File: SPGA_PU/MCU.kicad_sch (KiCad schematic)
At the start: 5 parts, among them U19 ESP32-S3-WROOM-1

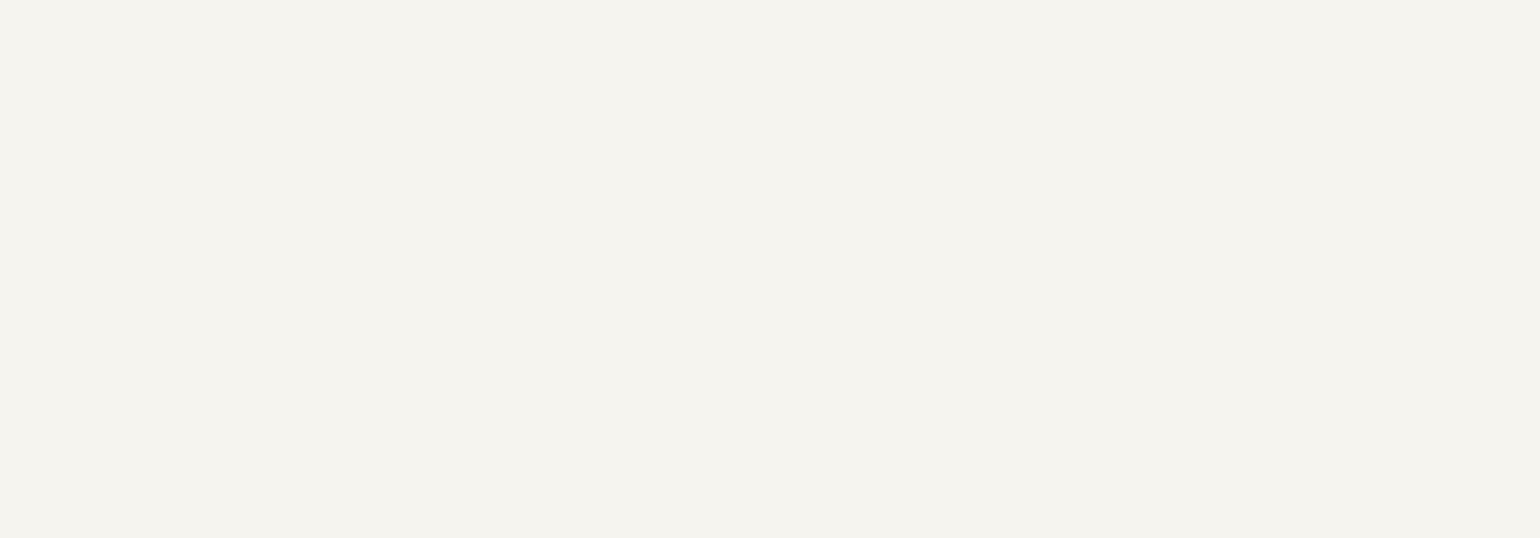
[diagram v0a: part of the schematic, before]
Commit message: thibgs
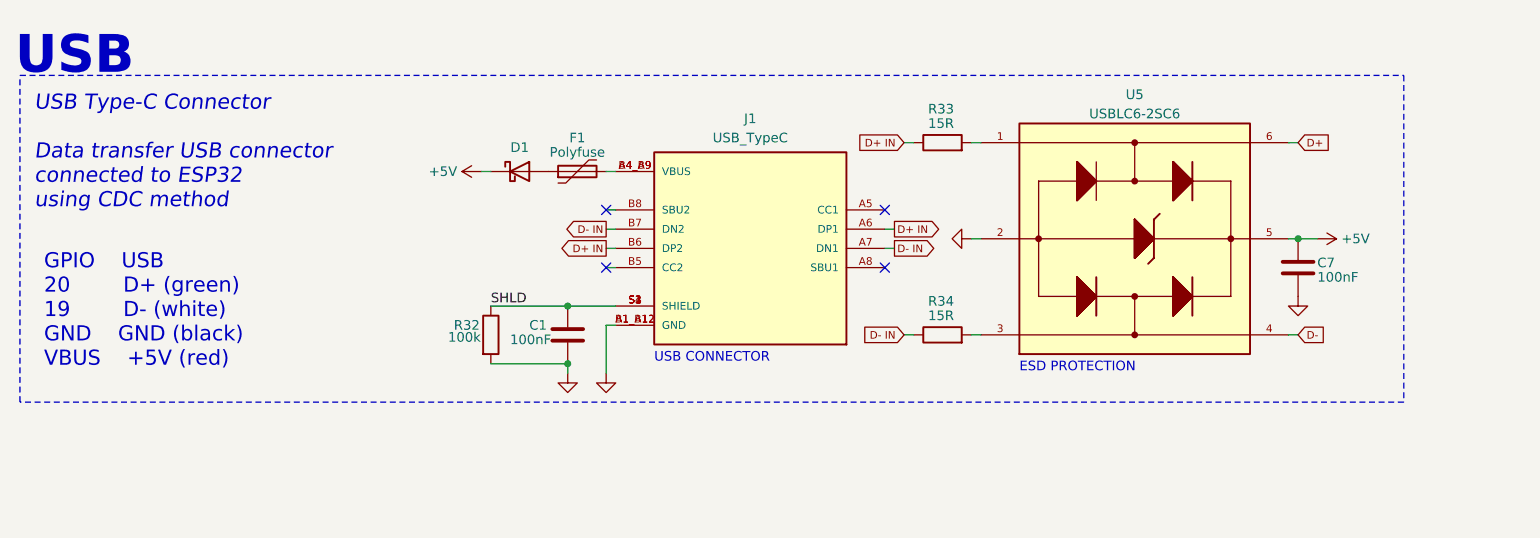
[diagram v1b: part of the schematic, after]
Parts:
- added C1, C7: 100nF, Capacitor_SMD:C_0805_2012Metric_Pad1.18x1.45mm_HandSolder, symbol Device:C
- added D1: D_Schottky, Diode_SMD:D_1206_3216Metric_Pad1.42x1.75mm_HandSolder, symbol Device:D_Schottky
- added F1: Polyfuse, Fuse:Fuse_0805_2012Metric, symbol Device:Polyfuse
- added J1: USB_TypeC, sumec_brd:HRO_TYPE-C-31-M-12, symbol sumec_sch_lib:USB_TypeC
- added R32: 100k, Resistor_SMD:R_0805_2012Metric_Pad1.20x1.40mm_HandSolder, symbol Device:R
- added R33, R34: 15R, Resistor_SMD:R_0805_2012Metric_Pad1.20x1.40mm_HandSolder, symbol Device:R
- added U5: USBLC6-2SC6, Package_TO_SOT_SMD:TSOT-23-6_HandSoldering, symbol sumec_library:USBLC6-2SC6
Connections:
- net GND: now also C1.1, C7.2, J1.A1_B12 (GND), J1.B1_A12 (GND), R32.2, U5.2
- new net: R33.2, U5.1
- new net: R34.2, U5.3
- new net: D1.2 (A), F1.1
- new net: F1.2, J1.A4_B9 (VBUS), J1.B4_A9 (VBUS)
- new net +5V: C7.1, D1.1 (K), U5.5
- new net D+: U5.6
- new net D+ IN: J1.A6 (DP1), J1.B6 (DP2), R33.1
- new net D-: U5.4
- new net D- IN: J1.A7 (DN1), J1.B7 (DN2), R34.1
- new net SHLD: C1.2, J1.S1 (SHIELD), J1.S2 (SHIELD), J1.S3 (SHIELD), J1.S4 (SHIELD), R32.1
- no-connect marks 4 -> 8
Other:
- note added: "ESD PROTECTION"
- note added: "GPIO USB 20 D+ (green) 19 D- (white) GND GND (black) VBUS +5V (red)"
- note added: "USB"
- note added: "USB CONNECTOR"
- note added: "USB Type-C Connector Data transfer USB connector connected to ESP32 using CDC method"
